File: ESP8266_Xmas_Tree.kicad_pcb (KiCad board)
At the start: 2 copper layers, 158.7 x 185.8 mm, 54 parts, among them U1 WeMos_D1_mini, U2 BMP280_Breakoutboard

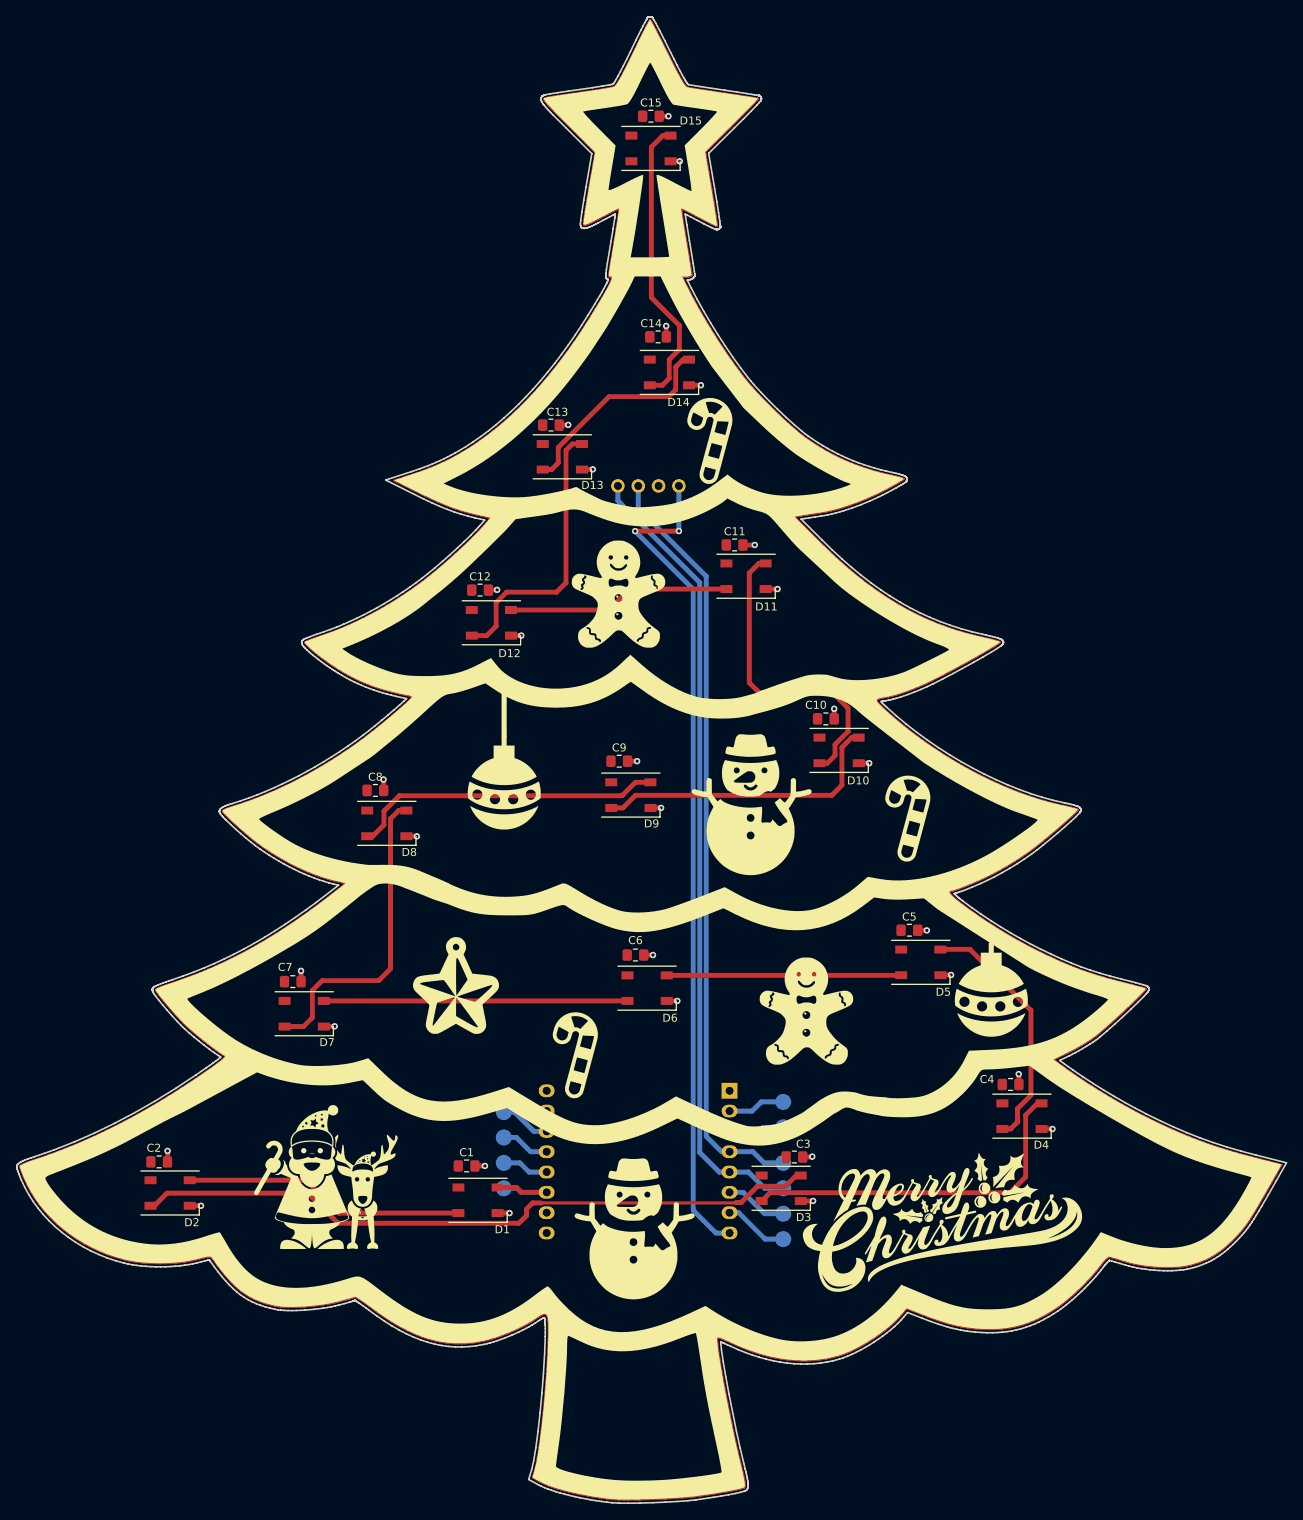
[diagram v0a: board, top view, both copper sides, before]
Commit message: adding README file
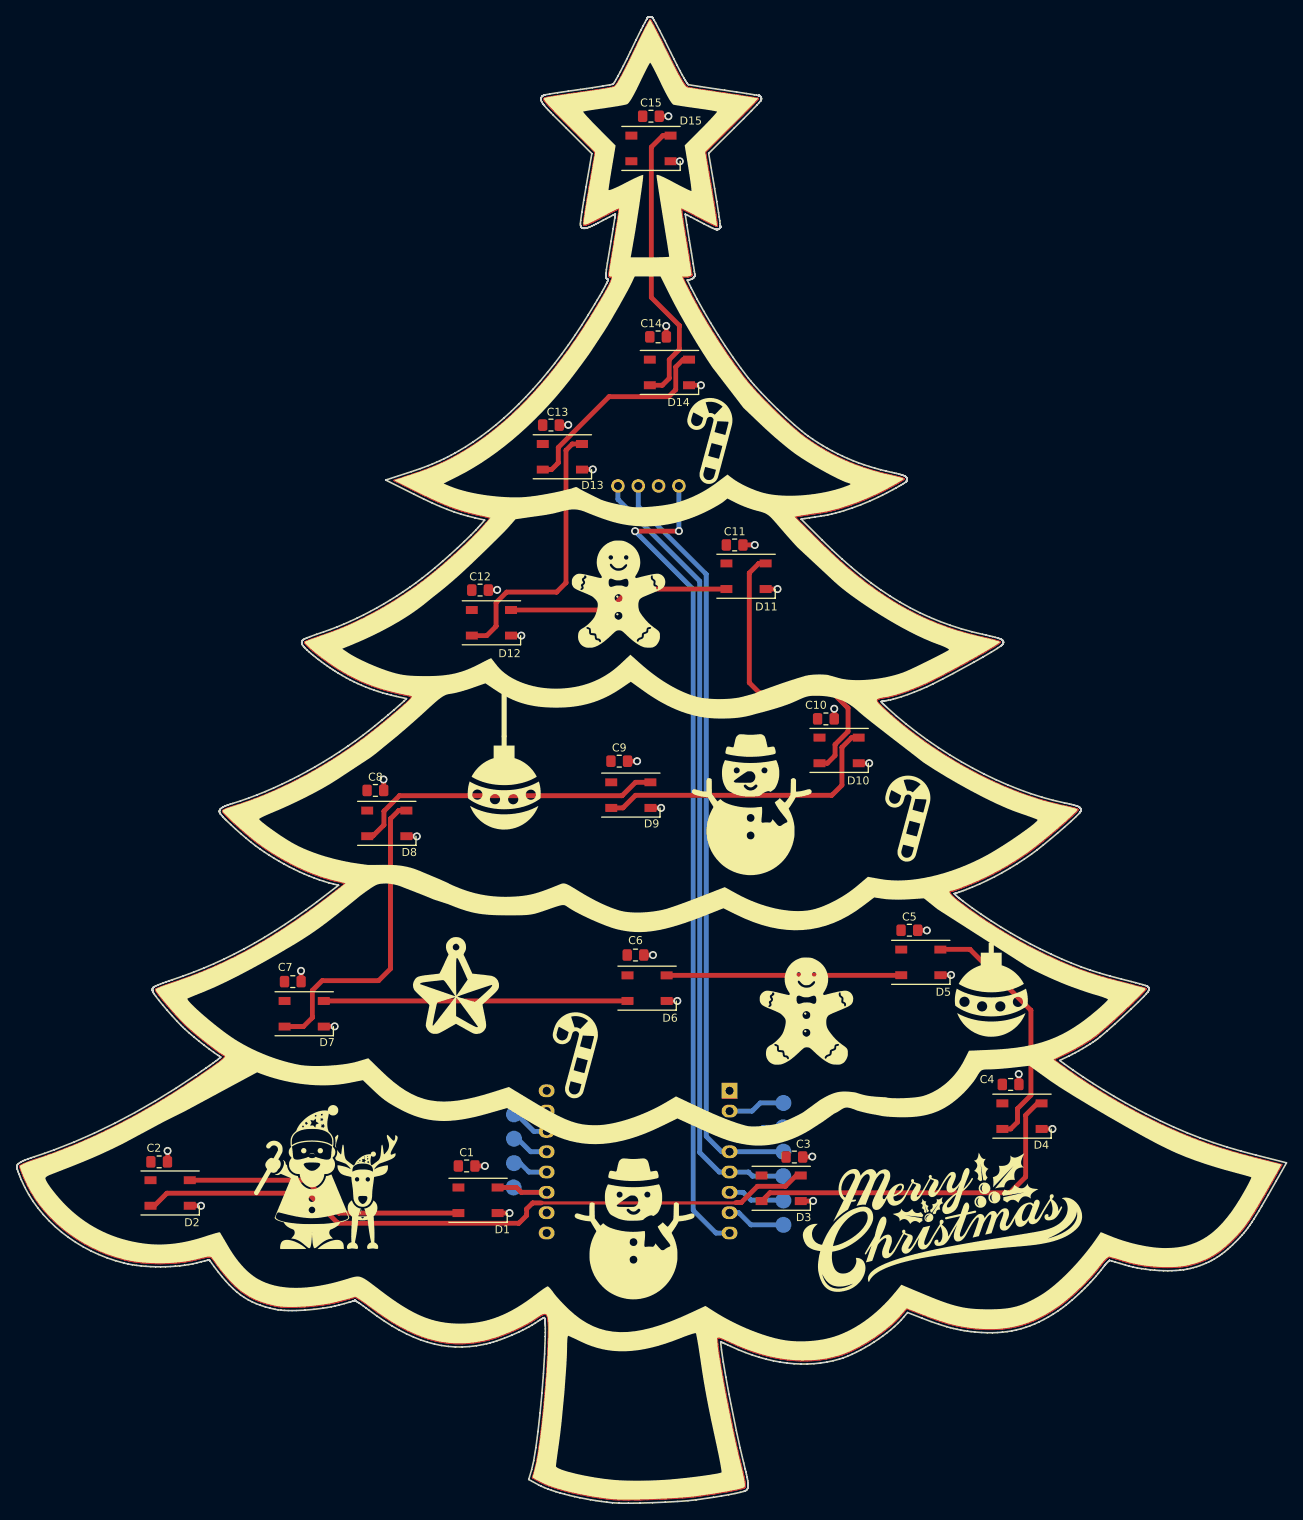
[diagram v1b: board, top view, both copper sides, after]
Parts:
- removed the REF** at (186.6, 128.5)
- added G***: LOGO, LOGO, B.Cu at (158.1, 189.1)
- added REF**: KiCad-Logo2_5mm_SilkScreen, Symbol:KiCad-Logo2_5mm_SilkScreen, B.Cu at (146.1, 193.3)
- moved REF** 2.19 mm to (170.5, 191.2)
- moved TP10 1.78 mm to (217.8, 202.7)
- moved TP9 1.65 mm to (217.8, 199.6)
- moved TP8 1.52 mm to (217.8, 196.6)
- moved TP7 1.40 mm to (217.8, 193.5)
- moved TP3 1.30 mm to (184.2, 188.9)
- moved TP4 1.28 mm to (184.2, 191.9)
- moved TP5 1.27 mm to (184.2, 195.0)
- moved TP6 1.22 mm to (184.1, 198.0)
- moved TP1 0.13 mm to (217.8, 187.5)
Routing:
- net Net-(TP3-Pad1): track 6.36 -> 4.97 mm
- net Net-(TP4-Pad1): track 6.09 -> 4.76 mm
- net Net-(TP5-Pad1): track 5.83 -> 4.55 mm
- net /WS2812B_DIN: track 12.0 -> 10.8 mm
- net Net-(TP10-Pad1): track 8.08 -> 7.36 mm
- net Net-(TP9-Pad1): track 7.81 -> 7.15 mm
- net /SDA: track 99.8 -> 99.2 mm
- net /SCL: track 95.8 -> 95.3 mm
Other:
- board text added: "ESP8266 Xmas Tree"
- board text added: "Rev 1.0.0-2022 by dokuhn and mancas"
